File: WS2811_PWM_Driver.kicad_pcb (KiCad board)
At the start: 2 copper layers, 43 parts, among them P1 Com, P2 PWM, P3 HS/LS, P4 HS/LS, P5 GND, P6 DIFIN, P7 DIFOUT, Q1 AO3401, Q2 AO3401, Q3 AO3401, Q4 AO3401, Q5 AO3401, Q6 AO3401, U1 SP485, U2 WS2811, U3 WS2811, U4 SP485

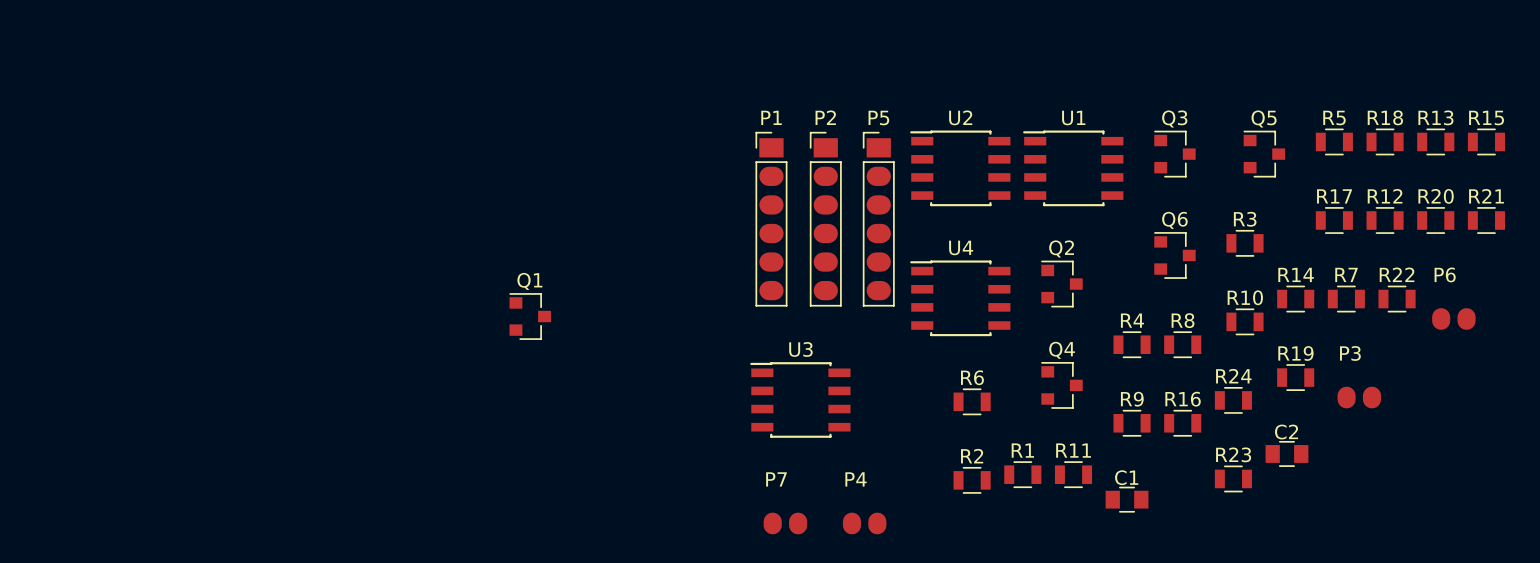
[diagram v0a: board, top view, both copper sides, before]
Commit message: PCB Update
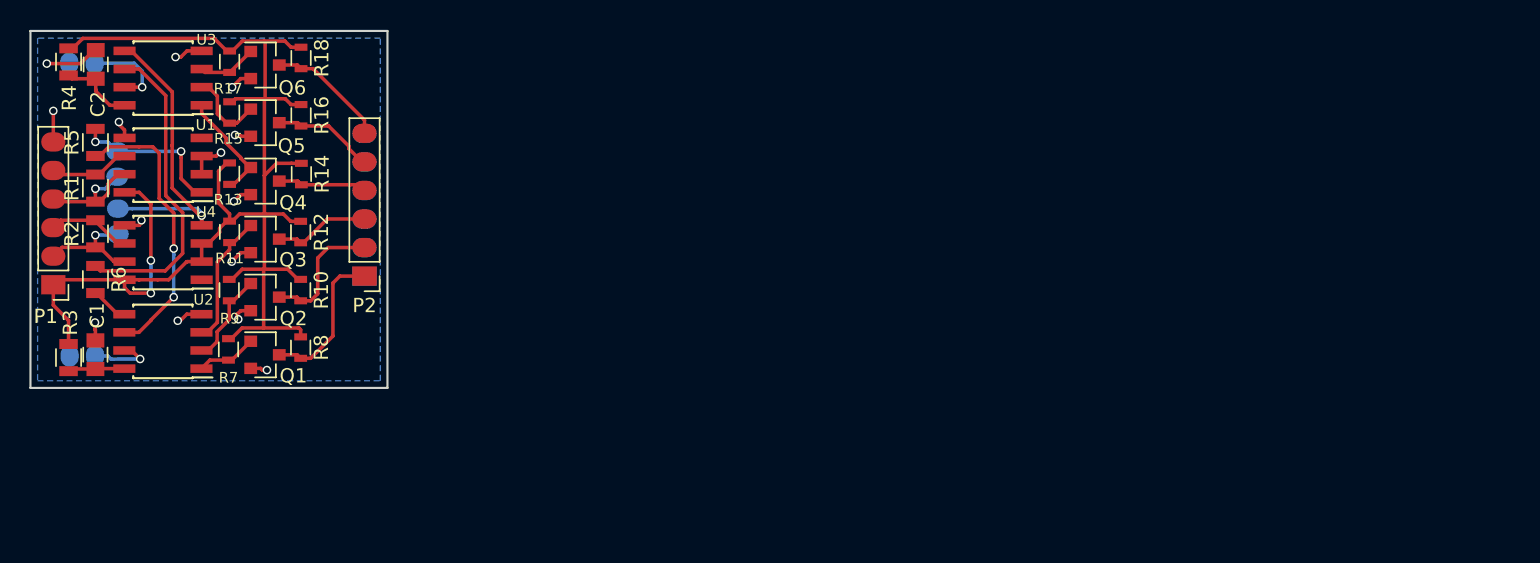
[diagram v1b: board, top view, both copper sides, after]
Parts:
- removed R19, R20, R21, R22, R23, R24: 510, Resistors_SMD:R_0805
- P3, P4, P5, P6, P7: moved to B.Cu
- Q1, Q2, Q3, Q4, Q5, Q6: value AO3401 -> MMBT4401; footprint PCB FootPrints:SOT-23 -> WS2811_PWM_PCB:SOT-23
- R10, R12, R8: value 33 -> 510; footprint Resistors_SMD:R_0805 -> Resistors_SMD:R_0603
- R11, R7, R9: value 33 -> 4K7; footprint Resistors_SMD:R_0805 -> Resistors_SMD:R_0603
- R13, R15, R17: value 330 -> 4K7; footprint Resistors_SMD:R_0805 -> Resistors_SMD:R_0603
- R14, R16, R18: value 330 -> 510; footprint Resistors_SMD:R_0805 -> Resistors_SMD:R_0603
- moved P6 94.2 mm to (106.1, 109.3), turned to 270 degrees
- moved P3 89.5 mm to (103.6, 122.8)
- moved R15 88.0 mm to (113.9, 105.7), turned to 270 degrees
- moved C2 87.8 mm to (104.6, 102.3), turned to 90 degrees
- moved R5 86.8 mm to (104.5, 107.8), turned to 90 degrees
- moved R13 84.5 mm to (113.9, 110.0), turned to 270 degrees
- moved R3 82.8 mm to (102.7, 122.9), turned to 270 degrees
- moved R7 78.4 mm to (113.9, 122.3), turned to 270 degrees
- moved R17 78.2 mm to (113.9, 102.2), turned to 270 degrees
- moved R4 77.1 mm to (102.7, 102.2), turned to 270 degrees
- moved R18 76.1 mm to (118.9, 101.9), turned to 270 degrees
- moved R12 75.9 mm to (118.9, 114.1), turned to 270 degrees
- moved C1 73.0 mm to (104.5, 122.7), turned to 90 degrees
- moved R14 70.2 mm to (119.0, 110.0), turned to 270 degrees
- moved Q5 70.0 mm to (116.4, 106.4)
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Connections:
- P1 pad 2: /INB -> /OUTB
- P1 pad 3: /INA -> /OUTA
- P1 pad 4: /OUTB -> /INB
- P1 pad 5: /OUTA -> /INA
- Q1 pad 1: Net-(Q1-Pad1) -> /Out1
- Q1 pad 2: +5V -> GND
- Q2 pad 1: Net-(Q2-Pad1) -> /Out2
- Q2 pad 2: +5V -> GND
- Q3 pad 1: Net-(Q3-Pad1) -> /Out3
- Q3 pad 2: +5V -> GND
- Q4 pad 1: Net-(Q4-Pad1) -> /Out4
- Q4 pad 2: +5V -> GND
- Q5 pad 1: Net-(Q5-Pad1) -> /Out5
- Q5 pad 2: +5V -> GND
- Q6 pad 1: Net-(Q6-Pad1) -> /Out6
- Q6 pad 2: +5V -> GND
- R10 pad 1: Net-(Q4-Pad1) -> +5V
- R10 pad 2: +5V -> /PWM2
- R11 pad 1: Net-(Q5-Pad1) -> +5V
- R11 pad 2: +5V -> /Out3
- R12 pad 1: Net-(Q6-Pad1) -> +5V
- R12 pad 2: +5V -> /PWM3
- R13 pad 1: /Out1 -> +5V
- R13 pad 2: Net-(Q1-Pad1) -> /Out4
- R14 pad 1: /Out2 -> +5V
- R14 pad 2: Net-(Q2-Pad1) -> /PWM4
- R15 pad 1: /Out3 -> +5V
- R15 pad 2: Net-(Q3-Pad1) -> /Out5
- R16 pad 1: /Out4 -> +5V
- R16 pad 2: Net-(Q4-Pad1) -> /PWM5
- R17 pad 1: /Out5 -> +5V
- R17 pad 2: Net-(Q5-Pad1) -> /Out6
- R18 pad 1: /Out6 -> +5V
- R18 pad 2: Net-(Q6-Pad1) -> /PWM6
- R7 pad 1: Net-(Q1-Pad1) -> +5V
- R7 pad 2: +5V -> /Out1
- R8 pad 1: Net-(Q2-Pad1) -> +5V
- R8 pad 2: +5V -> /PWM1
- R9 pad 1: Net-(Q3-Pad1) -> +5V
- R9 pad 2: +5V -> /Out2
- U1 pad 4: Net-(U1-Pad4) -> (no net)
- U4 pad 1: Net-(U4-Pad1) -> (no net)
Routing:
- net +5V: track 0.00 -> 98.2 mm, vias 0 -> 2
- net GND: track 0.00 -> 24.8 mm, vias 0 -> 14
- net Net-(R6-Pad1): track 0.00 -> 22.0 mm
- net /DI3: track 0.00 -> 21.6 mm, vias 0 -> 1
- net Net-(R5-Pad1): track 0.00 -> 20.1 mm, vias 0 -> 2
- net /DI1: track 0.00 -> 10.9 mm, vias 0 -> 2
- net /PWM1: track 0.00 -> 10.6 mm
- net /Out3: track 0.00 -> 9.32 mm
- net /PWM2: track 0.00 -> 9.09 mm
- net /INB: track 0.00 -> 9.03 mm, vias 0 -> 1
- net /PWM6: track 0.00 -> 8.49 mm
- net /OUTB: track 0.00 -> 8.12 mm, vias 0 -> 1
- net /Out4: track 0.00 -> 7.78 mm
- net /PWM5: track 0.00 -> 7.21 mm
- net /PWM3: track 0.00 -> 6.76 mm
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- added copper zone on B.Cu, net GND
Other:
- board outline added: 25 x 25 mm

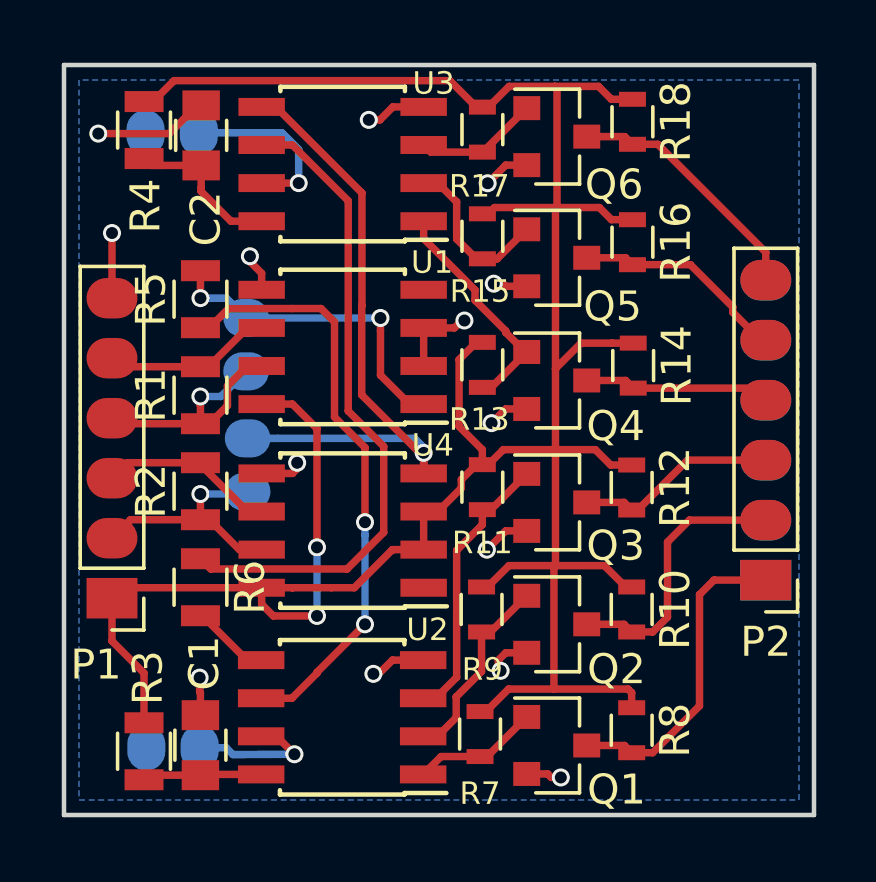
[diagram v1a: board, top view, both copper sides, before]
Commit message: PCB_Gerbers
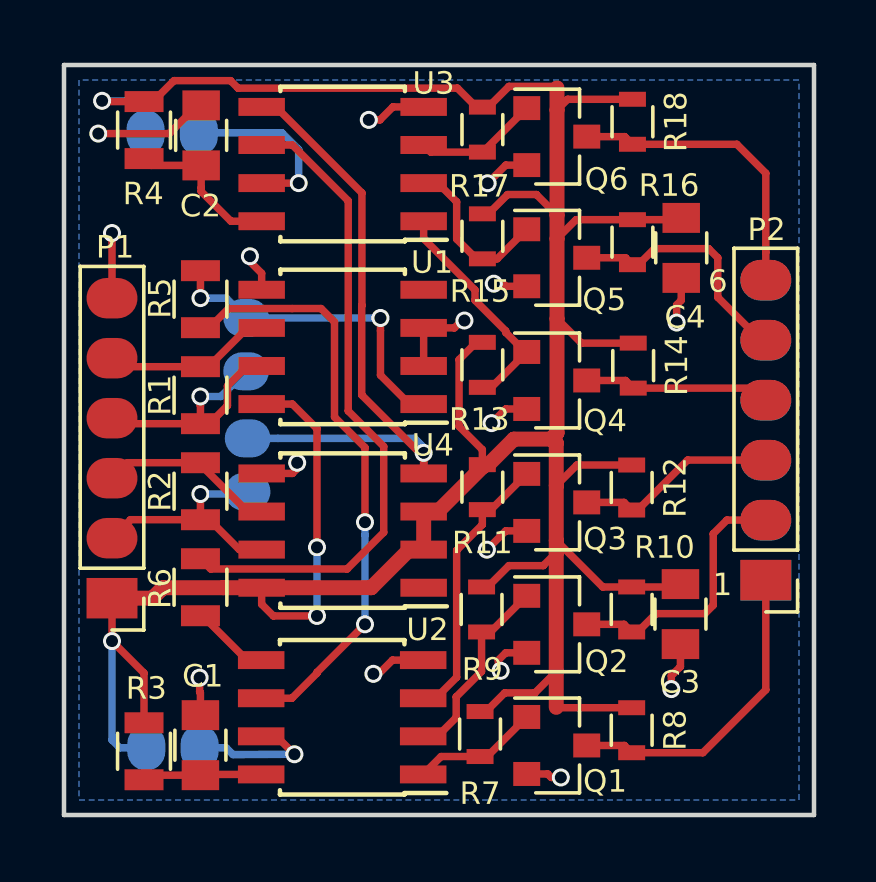
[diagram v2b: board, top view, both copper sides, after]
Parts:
- added C3: 10u/10V, Capacitors_SMD:C_0805, F.Cu at (120.5, 118.3)
- added C4: 10u/10V, Capacitors_SMD:C_0805, F.Cu at (120.6, 106.1)
- added REF***: KiCad-Logo2_6mm_SilkScreen, Symbols:KiCad-Logo2_6mm_SilkScreen, B.Cu at (115.4, 121.3)
- added REF***: OSHW-Logo_5.7x6mm_SilkScreen, Symbols:OSHW-Logo_5.7x6mm_SilkScreen, B.Cu at (119.1, 114.9)
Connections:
- P3 pad 1: GND -> +5V
- P4 pad 1: GND -> +5V
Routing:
- net +5V: track 98.2 -> 111.4 mm, vias 2 -> 4
- net GND: track 24.8 -> 28.0 mm, vias 14 -> 16
- net /PWM6: track 8.49 -> 10.0 mm
- net /PWM5: track 7.21 -> 8.32 mm
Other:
- board text added: "1"
- board text added: "5V"
- board text added: "6"
- board text added: "GND"
- board text added: "INA"
- board text added: "INB"
- board text added: "OUA"
- board text added: "OUB"
- board text added: "P3,P4-Open:HS Closed:LS"
- board text added: "P6,P7-Open:485 Closed:Direct"
- board text added: "PWM:400Hz/5V/5mA Power: 5V DC"
- board text added: "WS2811 6Ch PWM Driver V1.0 BK 2017"
